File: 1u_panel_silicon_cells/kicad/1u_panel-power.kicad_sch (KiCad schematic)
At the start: 70 parts, among them J1 MMS-104-01-[F/L]-SH, Q1 DMP3050LVT-7, Q2 DMP2240UDM-7, U10 TPS63060DSCR, U12 LTC4412, U3 LT1618EMSTRPBF, U4 INA226

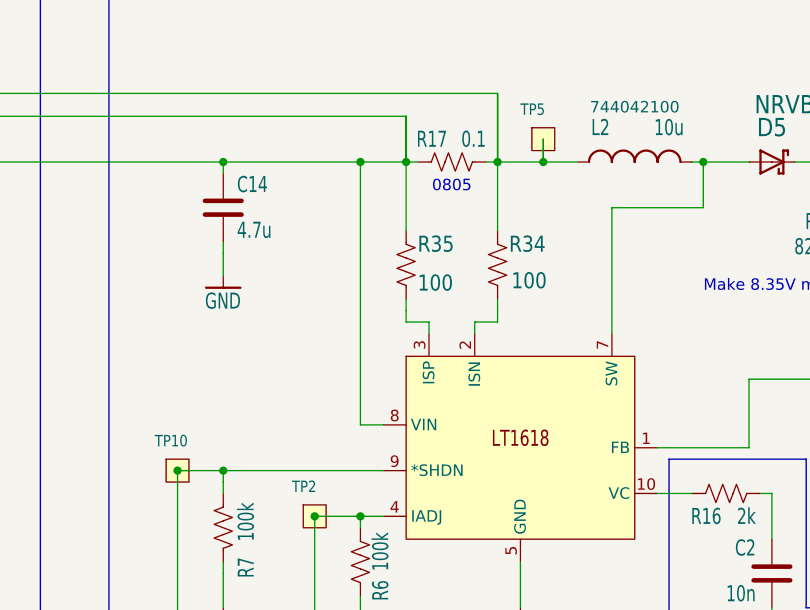
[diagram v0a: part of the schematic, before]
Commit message: final changes for silicon solar module
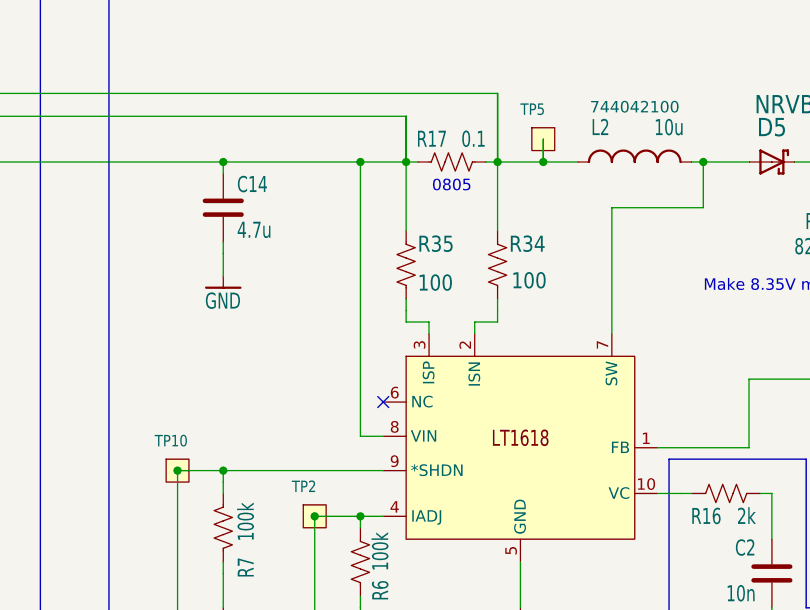
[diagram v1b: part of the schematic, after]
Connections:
- no-connect marks 0 -> 1
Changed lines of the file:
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@@
 		(color 0 0 0 0)
 	)
+	(no_connect
+		(at 180.34 86.36)
+	)
 	(polyline
 		(pts
@@
 	(wire
 		(pts
-			(xy 180.34 88.9) (xy 177.8 88.9)
+			(xy 180.34 90.17) (xy 177.8 90.17)
 		)
 		(stroke
@@
 	(wire
 		(pts
-			(xy 177.8 88.9) (xy 177.8 59.69)
+			(xy 177.8 90.17) (xy 177.8 59.69)
 		)
 		(stroke
@@
 		(pin "9"
 		)
+		(pin "6"
+		)
 		(instances
